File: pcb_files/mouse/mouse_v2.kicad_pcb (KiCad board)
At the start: 2 copper layers, 94.8 x 94.9 mm, 77 parts, among them J1 USB_C_Receptacle, J2 BT_Conn, J3 Conn_01x04_Female, J4 I2C_Conn, M1 Motor_DC, M2 Motor_DC, M3 CASTER_BALL, Q0 Q_Photo_NPN, Q1 Q_Photo_NPN, Q2 Q_Photo_NPN, Q3 Q_Photo_NPN, SW1 TL3315NF160Q, SW2 TL3315NF160Q, T0 Q_NMOS_DGS, T1 Q_NMOS_DGS, T2 Q_NMOS_DGS, T3 Q_NMOS_DGS, U1 Teensy3.2, U2 SN754410NE, U3 LM1084-5.0, U4 Encoder_3081, U5 Encoder_3081

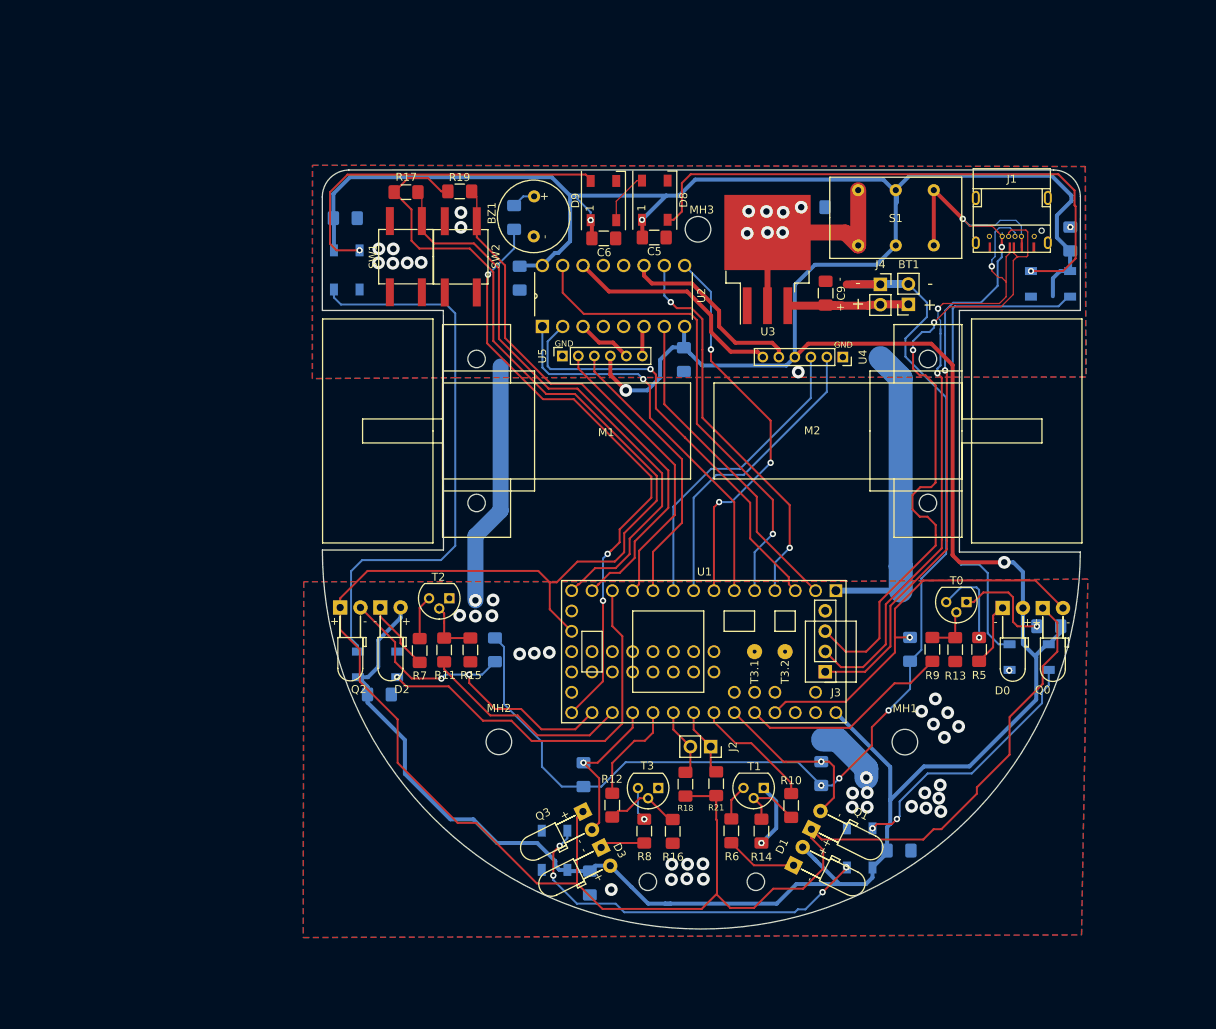
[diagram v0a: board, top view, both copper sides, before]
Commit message: Library updates
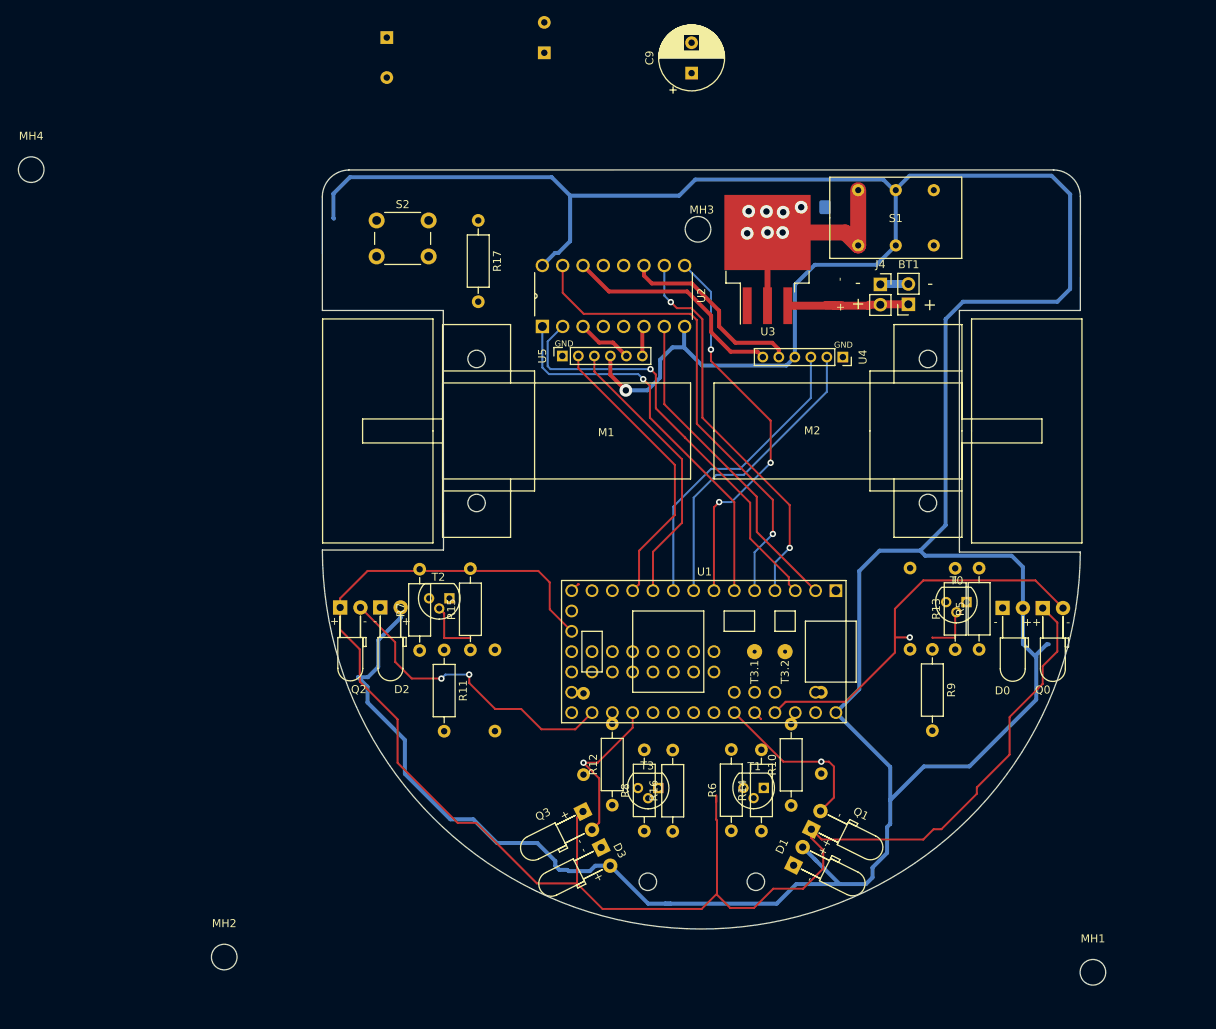
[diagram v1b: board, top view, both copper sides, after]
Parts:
- removed BZ1: Buzzer, misc:9x5.5mm Buzzer
- removed C1, C11, C12, C4, C5, C6, C7, C8: 0.1uF, Capacitor_SMD:C_1206_3216Metric_Pad1.42x1.75mm_HandSolder
- removed D10, D11, D4, D5, D6, D7, D8, D9: WS2812B, LED_SMD:LED_WS2812B_PLCC4_5.0x5.0mm_P3.2mm
- removed G***: LOGO, pika:magi800
- removed G***: LOGO, pika:magi1000
- removed G***: LOGO, pika:magi1200
- removed G***: LOGO, pika:magi1400
- removed J1: USB_C_Receptacle, misc:USB_C_REDUCED_PINS
- removed J2: BT_Conn, Connector_PinSocket_2.54mm:PinSocket_1x02_P2.54mm_Vertical
- removed J3: Conn_01x04_Female, Connector_PinHeader_2.54mm:PinHeader_1x04_P2.54mm_Vertical
- removed R18, R21: 4.7k, Resistor_SMD:R_1206_3216Metric_Pad1.42x1.75mm_HandSolder
- removed R19: R_PULL_UP, Resistor_SMD:R_1206_3216Metric_Pad1.42x1.75mm_HandSolder
- removed R20: R_BZ, Resistor_SMD:R_1206_3216Metric_Pad1.42x1.75mm_HandSolder
- removed SW1, SW2: TL3315NF160Q, misc:KSC_SW
- added MH4: M3, MountingHole:MountingHole_3.2mm_M3, F.Cu at (76.2, 54.6)
- added S2: GPTS203211B, Button_Switch_THT:SW_PUSH_6mm, F.Cu at (119.4, 61.0)
- C2, C9: footprint Capacitor_SMD:C_1206_3216Metric_Pad1.42x1.75mm_HandSolder -> Capacitor_THT:CP_Radial_D8.0mm_P3.80mm
- C3: footprint Capacitor_SMD:C_1206_3216Metric_Pad1.42x1.75mm_HandSolder -> Capacitor_THT:CP_Radial_D8.0mm_P5.00mm
- R1, R10, R11, R12, R13, R14, R15, R16, R17, R2, R3, R4, R5, R6, R7, R8, R9: footprint Resistor_SMD:R_1206_3216Metric_Pad1.42x1.75mm_HandSolder -> Resistor_THT:R_Axial_DIN0207_L6.3mm_D2.5mm_P10.16mm_Horizontal
- moved C3 54.8 mm to (120.7, 38.1)
- moved MH2 43.6 mm to (100.3, 153.0)
- moved MH1 37.2 mm to (208.9, 154.9)
- moved C9 32.2 mm to (158.8, 42.5)
- moved C2 28.3 mm to (140.3, 40.0), turned to 90 degrees
- moved R17 9.69 mm to (132.1, 61.0), turned to 270 degrees
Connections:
- S1 pad 3: /USB_VBUS -> /VUSB
- U1 pad 12: /RGB_DATA -> Net-(U1-Pad12)
- U1 pad 13: /PUSH_SW1 -> Net-(U1-Pad13)
- U1 pad 20: /Buzzer -> Net-(U1-Pad20)
- U1 pad 25: /i2c_SDA -> Net-(U1-Pad25)
- U1 pad 26: /i2c_SCL -> Net-(U1-Pad26)
- U1 pad 34: Net-(U1-Pad34) -> /VUSB
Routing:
- net /GND: track 240.9 -> 4.09 mm, vias 48 -> 0
- net /USB_VBUS: track 98.0 -> 0.00 mm, vias 3 -> 0
- net /3.3v: track 292.0 -> 203.1 mm
- net /USB_D+: track 83.0 -> 0.00 mm, vias 2 -> 0
- net /USB_D-: track 81.9 -> 0.00 mm, vias 3 -> 0
- net /Buzzer: track 76.7 -> 0.00 mm, vias 3 -> 0
- net /PUSH_SW: track 73.7 -> 1.24 mm
- net Net-(D7-Pad4): track 70.9 -> 0.00 mm, vias 1 -> 0
- net Net-(D10-Pad4): track 70.8 -> 0.00 mm
- net /PUSH_SW1: track 67.0 -> 0.00 mm
- net Net-(D6-Pad4): track 62.4 -> 0.00 mm
- net /RGB_DATA: track 49.5 -> 0.00 mm, vias 1 -> 0
- net Net-(D4-Pad4): track 47.6 -> 0.00 mm, vias 4 -> 0
- net Net-(D10-Pad2): track 44.4 -> 0.00 mm, vias 1 -> 0
- net Net-(D5-Pad4): track 33.3 -> 0.00 mm, vias 2 -> 0
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- removed copper zone on B.Cu, net /GND
- removed copper zone on F.Cu, net /GND

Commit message: Kit mouse before slimming
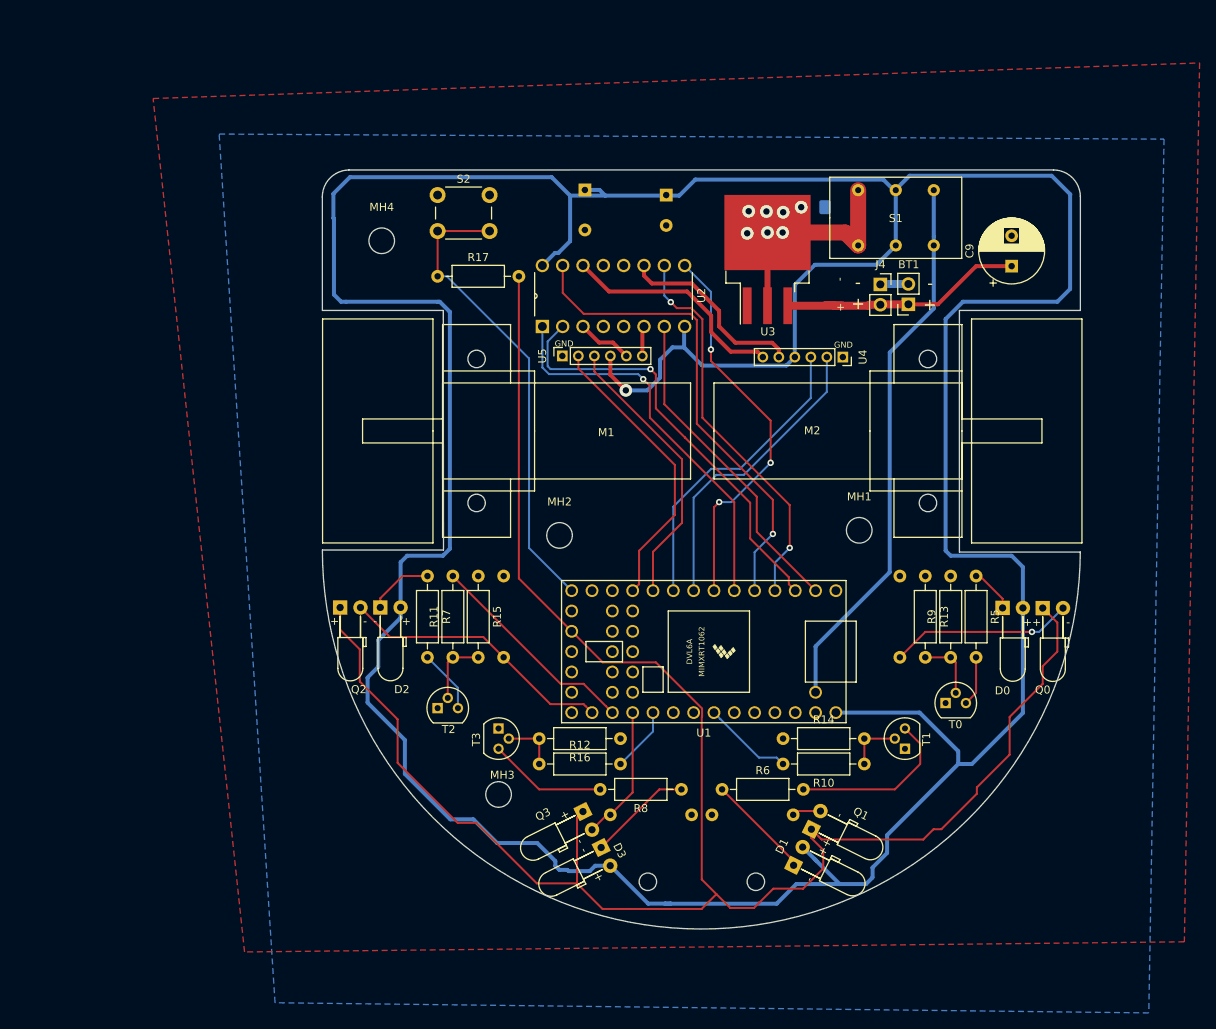
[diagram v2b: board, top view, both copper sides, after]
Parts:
- U1: value Teensy3.2 -> Teensy4.0; footprint teensy:Teensy30_31_32_LC -> teensy:Teensy40
- U3: value LM1084-5.0 -> LM1085-5.0
- moved MH3 74.9 mm to (134.6, 132.7)
- moved MH2 67.3 mm to (142.2, 100.3)
- moved MH1 62.5 mm to (179.7, 99.7)
- moved C9 46.7 mm to (198.8, 66.7)
- moved MH4 44.7 mm to (120.0, 63.5)
- moved C3 31.2 mm to (145.4, 57.1)
- moved C2 23.4 mm to (155.6, 57.8), turned to 270 degrees
- moved T3 21.3 mm to (134.6, 124.5), turned to 270 degrees
- moved T1 18.3 mm to (185.4, 127.0), turned to 90 degrees
- moved R2 14.6 mm to (161.3, 135.3), turned to 0 degrees
- moved R4 14.4 mm to (158.8, 135.3), turned to 180 degrees
- moved T2 13.8 mm to (127.0, 121.9), turned to 0 degrees
- moved R16 13.3 mm to (149.9, 125.7), turned to 180 degrees
- moved T0 12.9 mm to (190.5, 121.3), turned to 0 degrees
- moved R14 11.9 mm to (170.2, 125.7), turned to 0 degrees
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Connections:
- U1 pad 28: /Reciever_1 -> Net-(U1-Pad28)
- U1 pad 29: /Emitter_0 -> Net-(U1-Pad29)
- U1 pad 30: /Reciever_0 -> Net-(U1-Pad30)
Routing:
- net /VUSB: track 0.03 -> 68.9 mm
- net /PUSH_SW: track 1.24 -> 59.1 mm
- net /3.3v: track 203.1 -> 244.6 mm
- net /5v: track 445.2 -> 480.2 mm
- net /Emitter_2: track 0.00 -> 27.0 mm
- net /Reciever_0: track 49.4 -> 22.9 mm
- net Net-(R6-Pad2): track 0.00 -> 21.2 mm
- net /Reciever_1: track 21.5 -> 3.60 mm, vias 1 -> 0
- net /vBatt: track 17.3 -> 32.2 mm
- net Net-(R8-Pad2): track 0.00 -> 14.8 mm
- net Net-(D1-Pad1): track 0.00 -> 13.2 mm
- net Net-(D3-Pad1): track 0.80 -> 13.8 mm
- net /Emitter_1: track 0.00 -> 11.3 mm
- net Net-(D2-Pad1): track 0.00 -> 8.19 mm
- net /Emitter_3: track 0.00 -> 8.11 mm
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- added copper zone on B.Cu, net /GND
- added copper zone on F.Cu, net /GND
